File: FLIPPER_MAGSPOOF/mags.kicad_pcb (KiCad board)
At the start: 2 copper layers, 67 x 23.3 mm, 25 parts, among them J1 Coil, J2 Conn_01x10_Socket, J3 Conn_01x08_Socket, J4 Conn_01x08_Socket, J5 Conn_01x10_Socket, U1 TC4424

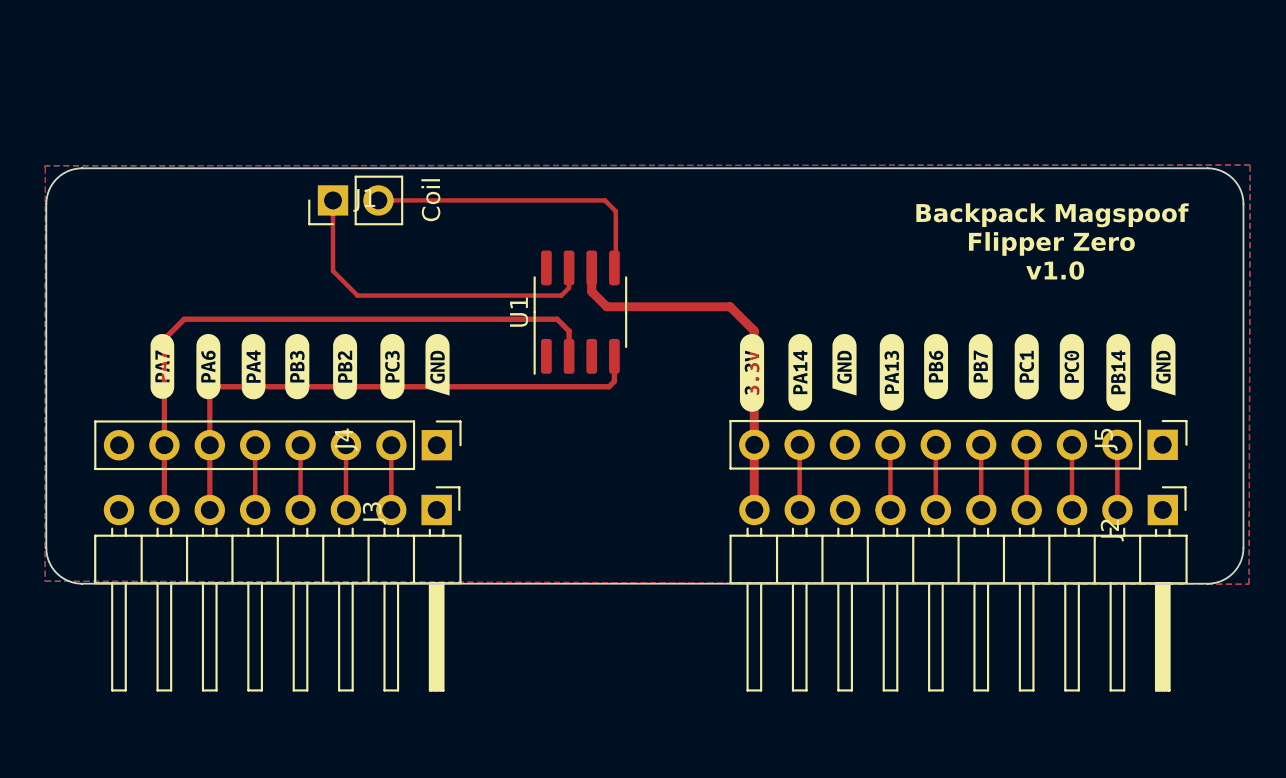
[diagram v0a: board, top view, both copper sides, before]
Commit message: Move_Pins
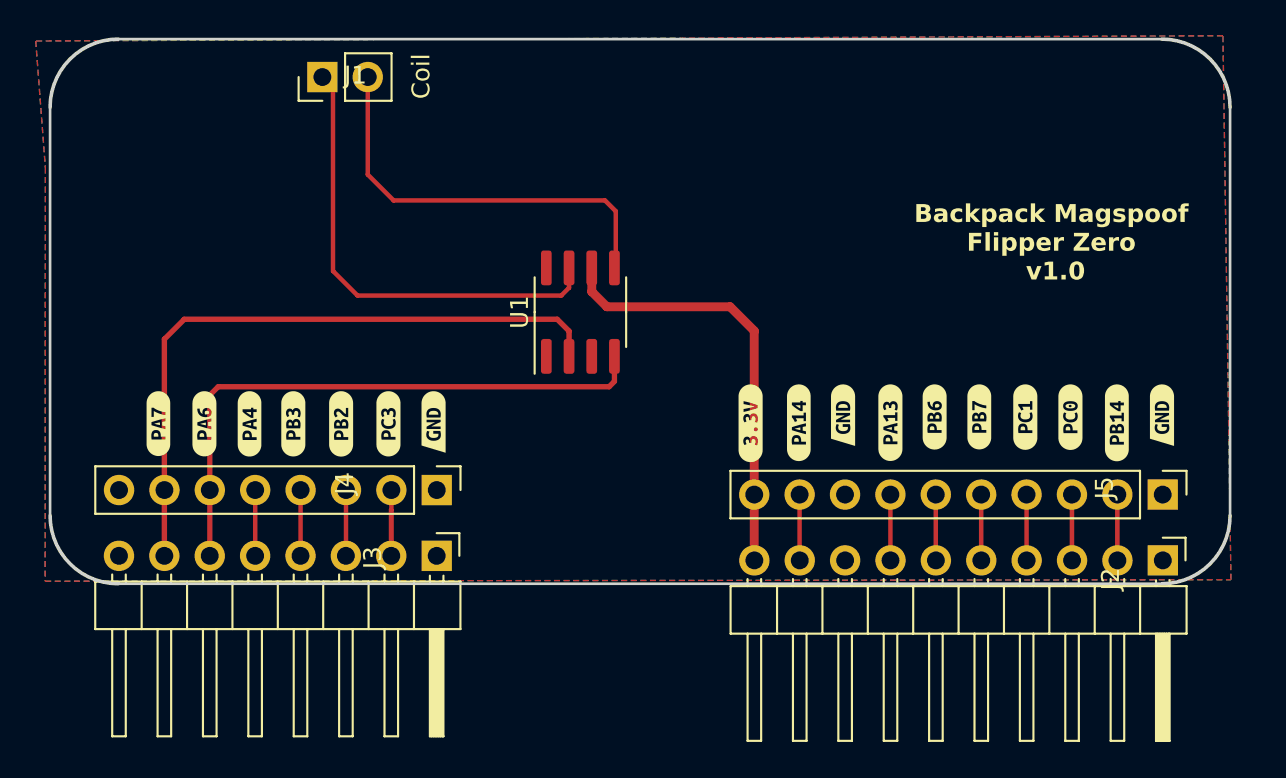
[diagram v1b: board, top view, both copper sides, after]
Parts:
- moved J1 6.93 mm to (211.5, 58.3)
- moved kibuzzard-6488EEAF 3.21 mm to (217.7, 77.6)
- moved kibuzzard-648B91CB 3.21 mm to (207.4, 77.7)
- moved kibuzzard-648B91E6 3.21 mm to (209.8, 77.7)
- moved kibuzzard-648B91FC 3.21 mm to (212.5, 77.7)
- moved kibuzzard-648B921B 3.21 mm to (215.2, 77.7)
- moved kibuzzard-648B922F 3.21 mm to (202.3, 77.7)
- moved kibuzzard-648B923F 3.21 mm to (204.9, 77.7)
- moved kibuzzard-6488EEAF 2.82 mm to (240.6, 77.2)
- moved kibuzzard-6488F75A 2.82 mm to (235.4, 77.7)
- moved kibuzzard-648B93D2 2.82 mm to (248.2, 77.3)
- moved kibuzzard-648B93E0 2.82 mm to (245.7, 77.3)
- moved kibuzzard-648B93EF 2.82 mm to (250.8, 77.3)
- moved kibuzzard-648B9401 2.82 mm to (253.3, 77.3)
- moved kibuzzard-648B9410 2.82 mm to (255.9, 77.6)
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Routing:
- net /Out_A: track 19.0 -> 26.2 mm
- net /Out_B: track 16.7 -> 23.4 mm
- net +3V3: track 21.4 -> 24.2 mm
- net /PC3: track 3.64 -> 6.26 mm
- net /IN_B: track 30.8 -> 33.4 mm
- net /IN_A: track 34.4 -> 36.9 mm
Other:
- board size 67 x 23.3 mm -> 66 x 30.5 mm
- rule pad_to_mask_clearance: 0 -> 0.051
